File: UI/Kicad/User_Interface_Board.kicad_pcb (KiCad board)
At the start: 2 copper layers, 71 x 62.8 mm, 13 parts, among them J1 BHR-16-HUA, J2 Conn_01x02_Male, J3 Conn_01x02_Male, J4 Conn_01x02_Male, J5 Conn_01x02_Male, J6 Conn_01x08_Male, J7 Conn_01x05_Male, J8 Conn_01x03_Male

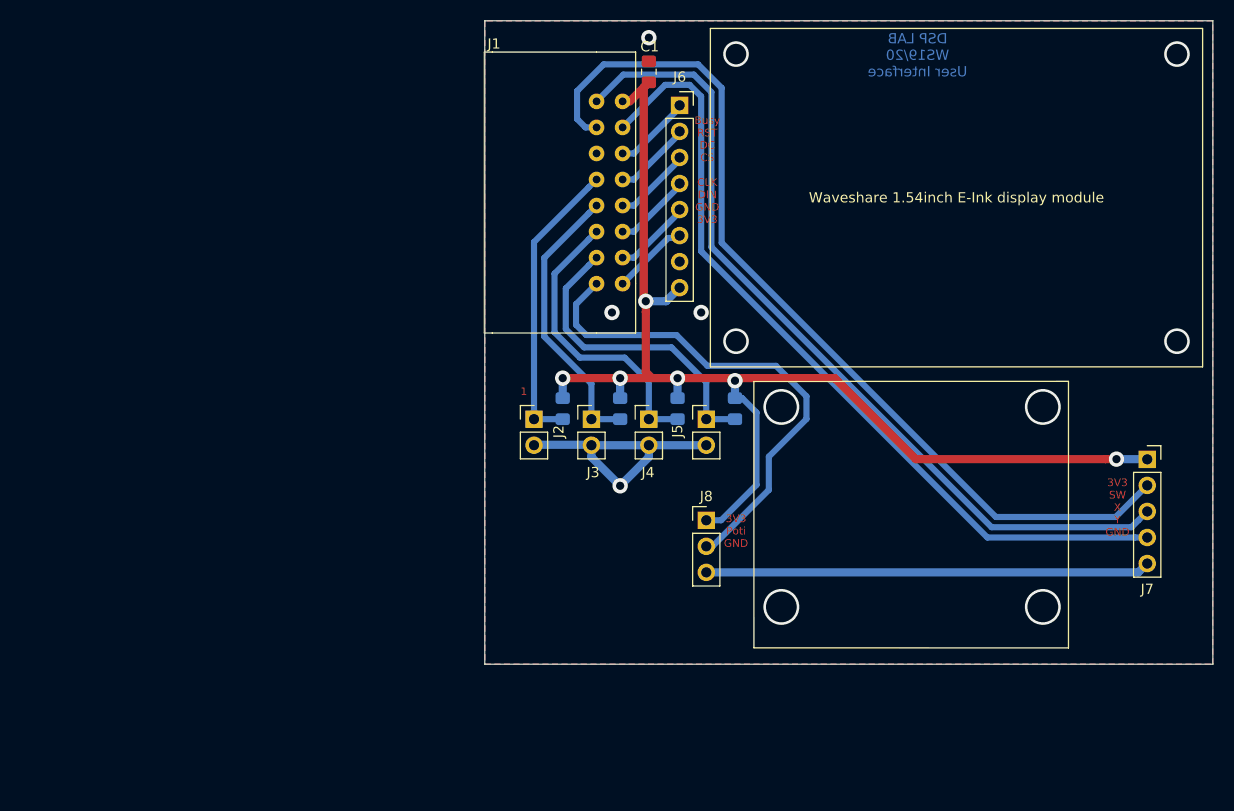
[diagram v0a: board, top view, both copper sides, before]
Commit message: Display-Board Updated!
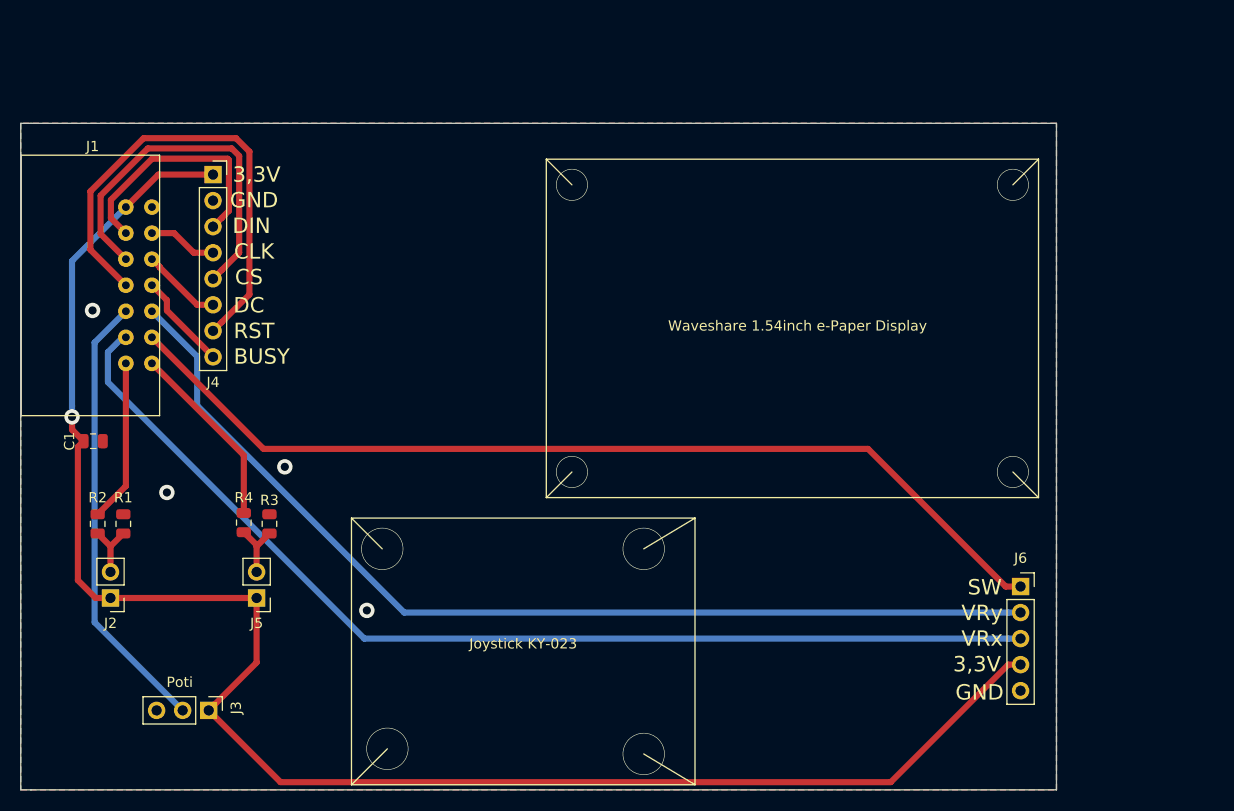
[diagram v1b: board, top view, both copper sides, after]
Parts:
- removed J7: Conn_01x05_Male, Connector_PinSocket_2.54mm:PinSocket_1x05_P2.54mm_Vertical
- removed J8: Conn_01x03_Male, Connector_PinHeader_2.54mm:PinHeader_1x03_P2.54mm_Vertical
- C1: value 1uF -> 1u; footprint Resistor_SMD:R_0805_2012Metric_Pad1.15x1.40mm_HandSolder -> Capacitor_SMD:C_0805_2012Metric
- J1: value BHR-16-HUA -> BHR-14-HUA; footprint User_Interface_Board:BHR-16-HUA -> User_Interface_Board:BHR-14-HUA
- J3: value Conn_01x02_Male -> Conn_01x03_Male; footprint Connector_PinHeader_2.54mm:PinHeader_1x02_P2.54mm_Vertical -> Connector_PinHeader_2.54mm:PinHeader_1x03_P2.54mm_Vertical
- J4: value Conn_01x02_Male -> Conn_01x08_Male; footprint Connector_PinHeader_2.54mm:PinHeader_1x02_P2.54mm_Vertical -> Connector_PinSocket_2.54mm:PinSocket_1x08_P2.54mm_Vertical
- J6: value Conn_01x08_Male -> Conn_01x05_Male; footprint Connector_PinSocket_2.54mm:PinSocket_1x08_P2.54mm_Vertical -> Connector_PinSocket_2.54mm:PinSocket_1x05_P2.54mm_Vertical
- R1, R3: value 10k -> 100k; footprint Resistor_SMD:R_0805_2012Metric_Pad1.15x1.40mm_HandSolder -> Resistor_SMD:R_0805_2012Metric; moved to F.Cu
- R2, R4: value 10k -> 220; footprint Resistor_SMD:R_0805_2012Metric_Pad1.15x1.40mm_HandSolder -> Resistor_SMD:R_0805_2012Metric; moved to F.Cu
- moved C1 65.1 mm to (89.8, 103.2), turned to 0 degrees
- moved J6 57.5 mm to (180.2, 117.4)
- moved R2 52.2 mm to (90.2, 111.3)
- moved R4 49.2 mm to (104.5, 111.2)
- moved J1 49.1 mm to (90.7, 88.1)
- moved J4 48.7 mm to (101.5, 77.2)
- moved J5 47.2 mm to (105.8, 118.5), turned to 180 degrees
- moved J3 46.9 mm to (101.1, 129.5), turned to 270 degrees
- moved J2 44.8 mm to (91.5, 118.5), turned to 180 degrees
- moved R1 44.3 mm to (92.8, 111.3), turned to 90 degrees
- moved R3 41.4 mm to (107.0, 111.3), turned to 90 degrees
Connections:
- C1 pad 1: /+3,3V -> /3,3V
- J1 pad 1: /Poti -> /3,3V
- J1 pad 10: /CLK -> /VRy
- J1 pad 11: /CS -> /VRx
- J1 pad 12: /DC -> /SW
- J1 pad 13: /RST -> /BACK_BUTTON
- J1 pad 14: /Busy -> /ENTER_BUTTON
- J1 pad 2: /Button4 -> GND
- J1 pad 3: /Button3 -> /DIN
- J1 pad 4: /Button2 -> /CLK
- J1 pad 5: /Button1 -> /CS
- J1 pad 6: GND -> /DC
- J1 pad 7: /SW -> /RST
- J1 pad 8: /X -> /BUSY
- J1 pad 9: /DIN -> /POTI
- J2 pad 1: /Button1 -> /3,3V
- J2 pad 2: GND -> Net-(J2-Pad2)
- J3 pad 1: /Button2 -> /3,3V
- J3 pad 2: GND -> /POTI
- J4 pad 1: /Button3 -> /3,3V
- J5 pad 1: /Button4 -> /3,3V
- J5 pad 2: GND -> Net-(J5-Pad2)
- J6 pad 1: /Busy -> /SW
- J6 pad 2: /RST -> /VRy
- J6 pad 3: /DC -> /VRx
- J6 pad 4: /CS -> /3,3V
- J6 pad 5: /CLK -> GND
- R1 pad 1: /+3,3V -> Net-(J2-Pad2)
- R1 pad 2: /Button1 -> GND
- R2 pad 1: /+3,3V -> /BACK_BUTTON
- R2 pad 2: /Button2 -> Net-(J2-Pad2)
- R3 pad 1: /+3,3V -> Net-(J5-Pad2)
- R3 pad 2: /Button3 -> GND
- R4 pad 1: /+3,3V -> /ENTER_BUTTON
- R4 pad 2: /Button4 -> Net-(J5-Pad2)
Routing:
- net /3,3V: track 0.00 -> 166.9 mm, vias 0 -> 1
- net /+3,3V: track 120.7 -> 0.00 mm, vias 6 -> 0
- net /VRx: track 0.00 -> 104.6 mm
- net /VRy: track 0.00 -> 99.7 mm
- net /X: track 82.5 -> 0.00 mm
- net /Y: track 80.0 -> 0.00 mm
- net GND: track 70.5 -> 0.00 mm
- net /Poti: track 49.2 -> 0.00 mm
- net /POTI: track 0.00 -> 43.7 mm
- net /RST: track 7.64 -> 47.7 mm
- net /Button4: track 30.5 -> 0.00 mm
- net /Button3: track 29.2 -> 0.00 mm
- net /Button1: track 28.7 -> 0.00 mm
- net /CS: track 7.64 -> 36.0 mm
- net /Button2: track 27.9 -> 0.00 mm
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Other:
- board size 71 x 62.8 mm -> 101 x 65 mm
- board text added: "3,3V"
- board text added: "BUSY"
- board text added: "CLK"
- board text added: "CS"
- board text added: "DC"
- board text added: "DIN"
- board text added: "DSP-Projekt SS 2021 GUI-Board"
- board text added: "GND"
- board text added: "Joystick KY-023"
- board text added: "Poti"
- board text added: "RST"
- board text added: "SW"
- board text added: "VRx"
- board text added: "VRy"
- board text added: "Waveshare 1.54inch e-Paper Display"
- board text removed: "1"
- board text removed: "3V3 Poti GND"
- board text removed: "3V3 SW X Y GND"
- board text removed: "Busy RST DC CS CLK DIN GND 3V3"
- board text removed: "DSP LAB WS19/20 User Interface"
- board text removed: "Waveshare 1.54inch E-Ink display module"
